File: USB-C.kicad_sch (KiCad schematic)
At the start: 3 parts, among them J3 CX90M-16P

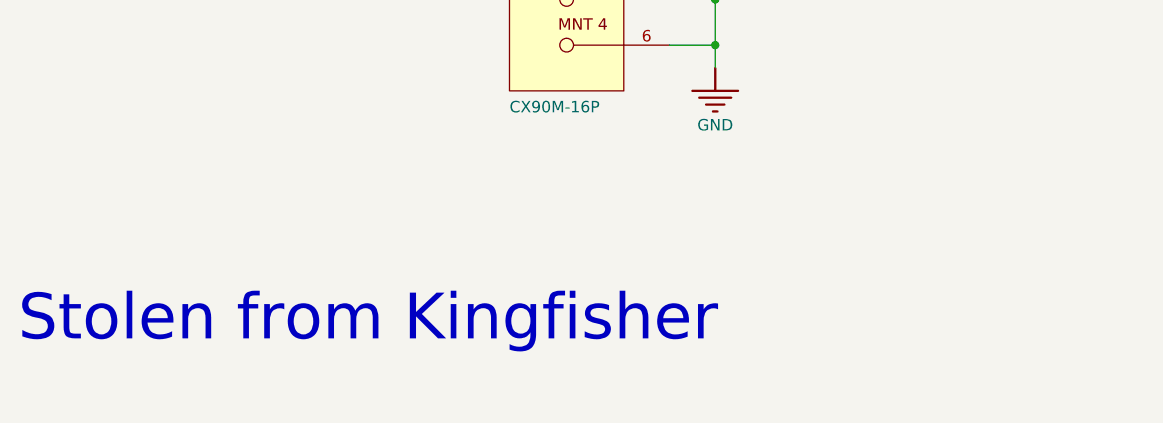
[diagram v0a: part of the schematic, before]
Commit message: Initial library setup
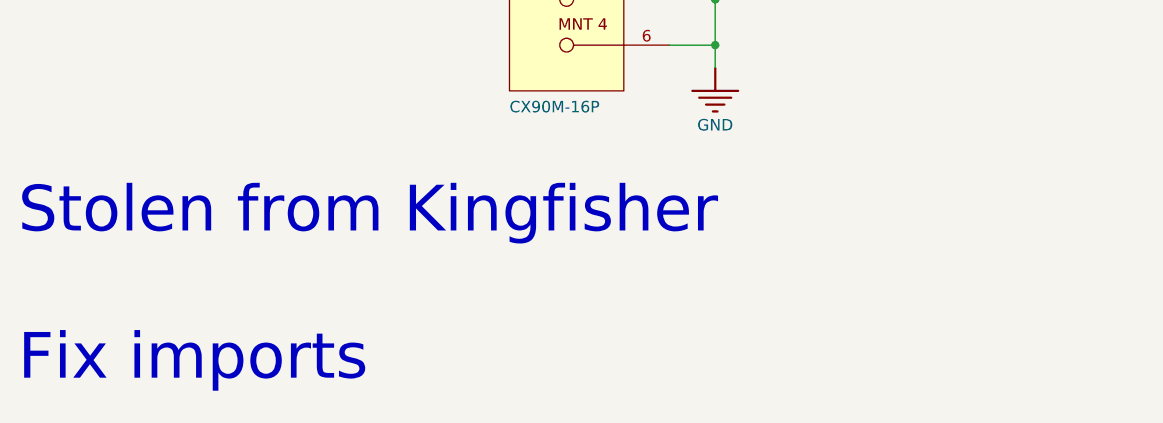
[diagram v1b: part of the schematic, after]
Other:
- note added: "Stolen from Kingfisher Fix imports"
- note removed: "Stolen from Kingfisher"
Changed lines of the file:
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@@
 	(generator_version "10.0")
 	(paper "A4")
-	(text "Stolen from Kingfisher\n"
+	(text "Stolen from Kingfisher\n\nFix imports"
 		(exclude_from_sim no)
-		(at 25.4 182.88 0)
+		(at 25.4 179.07 0)
 		(effects
 			(font

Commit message: Revert "Temporary save if I accidentally bust something"
This reverts commit 974f20a02fde00668d4b3d45f60811623d130148.
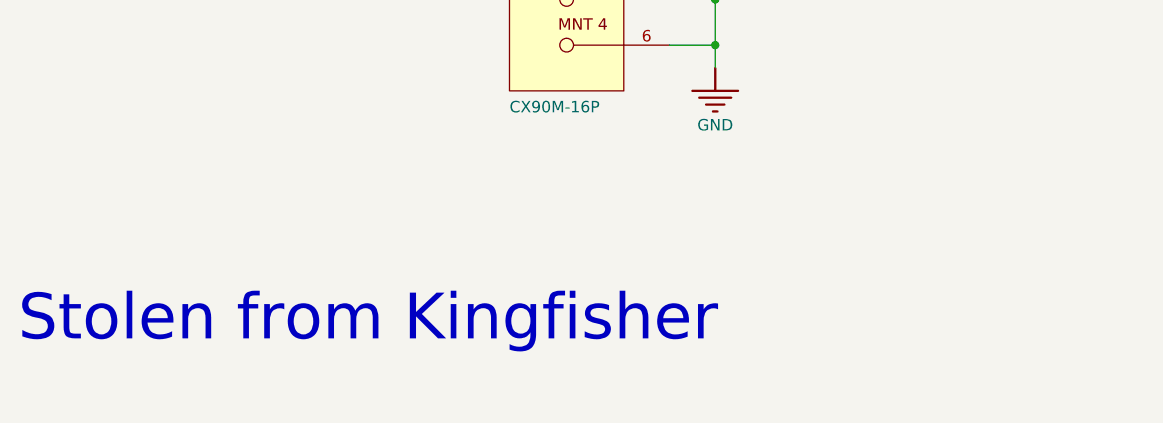
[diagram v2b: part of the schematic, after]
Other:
- note added: "Stolen from Kingfisher"
- note removed: "Stolen from Kingfisher Fix imports"
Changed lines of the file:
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@@
 	(generator_version "10.0")
 	(paper "A4")
-	(text "Stolen from Kingfisher\n\nFix imports"
+	(text "Stolen from Kingfisher\n"
 		(exclude_from_sim no)
-		(at 25.4 179.07 0)
+		(at 25.4 182.88 0)
 		(effects
 			(font
